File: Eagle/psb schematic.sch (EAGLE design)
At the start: 12 parts, among them J1 CONN_26X2

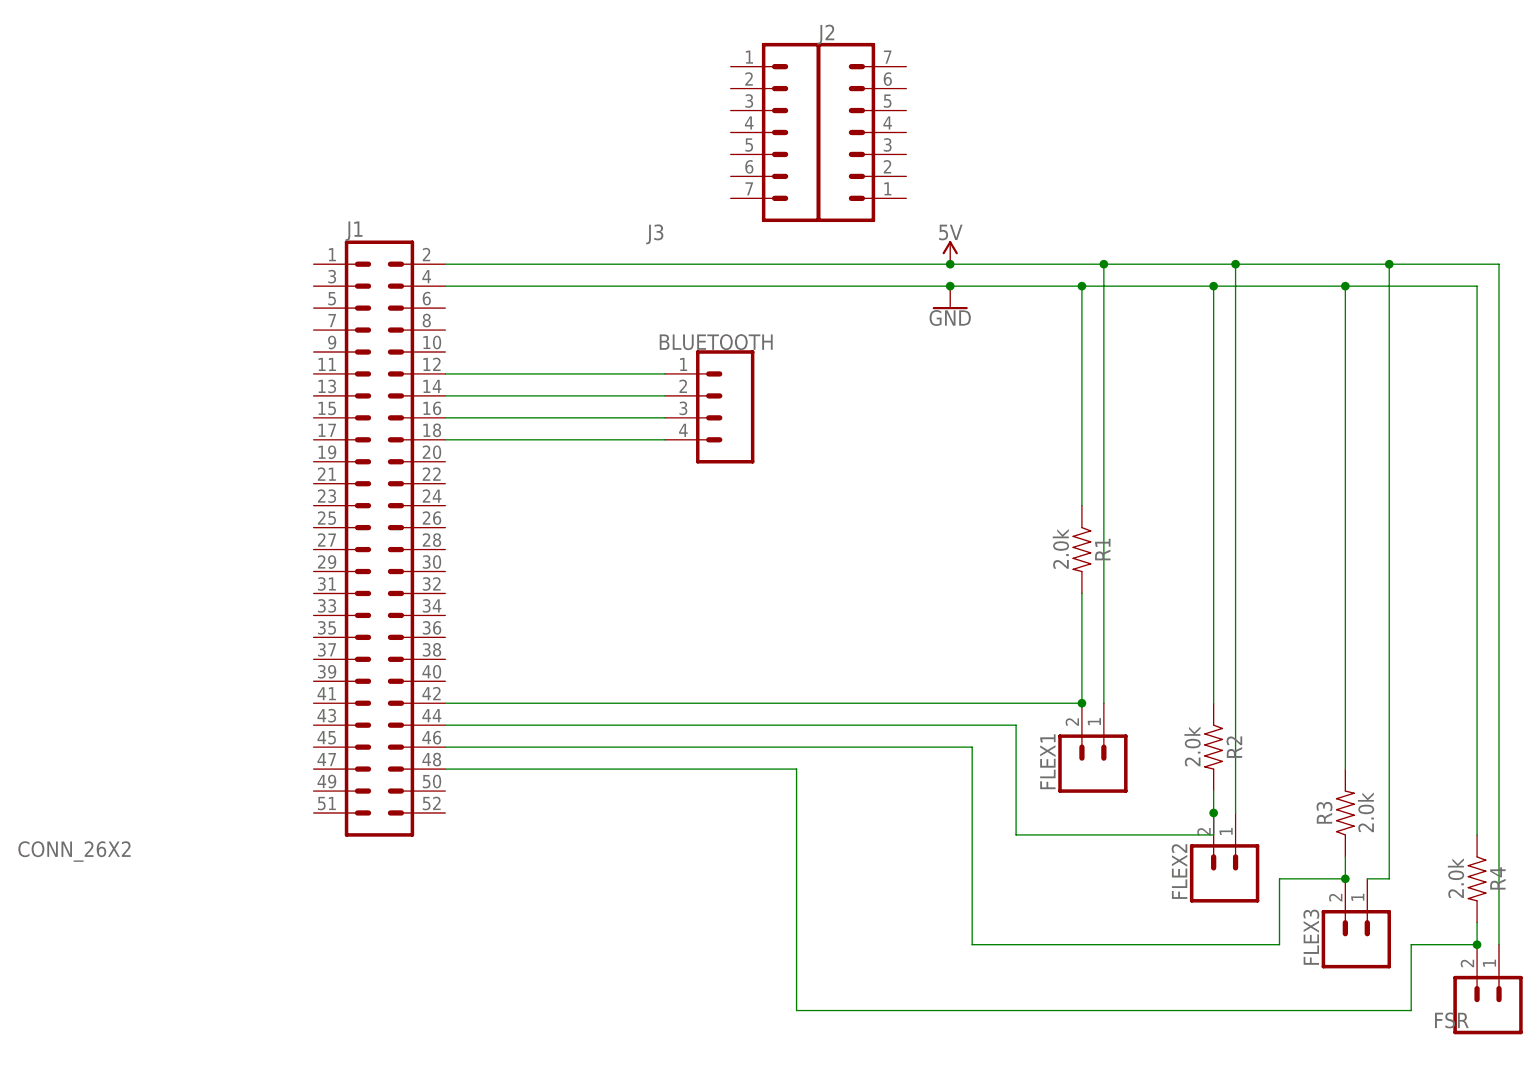
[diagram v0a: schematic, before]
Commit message: Correzioni PCB
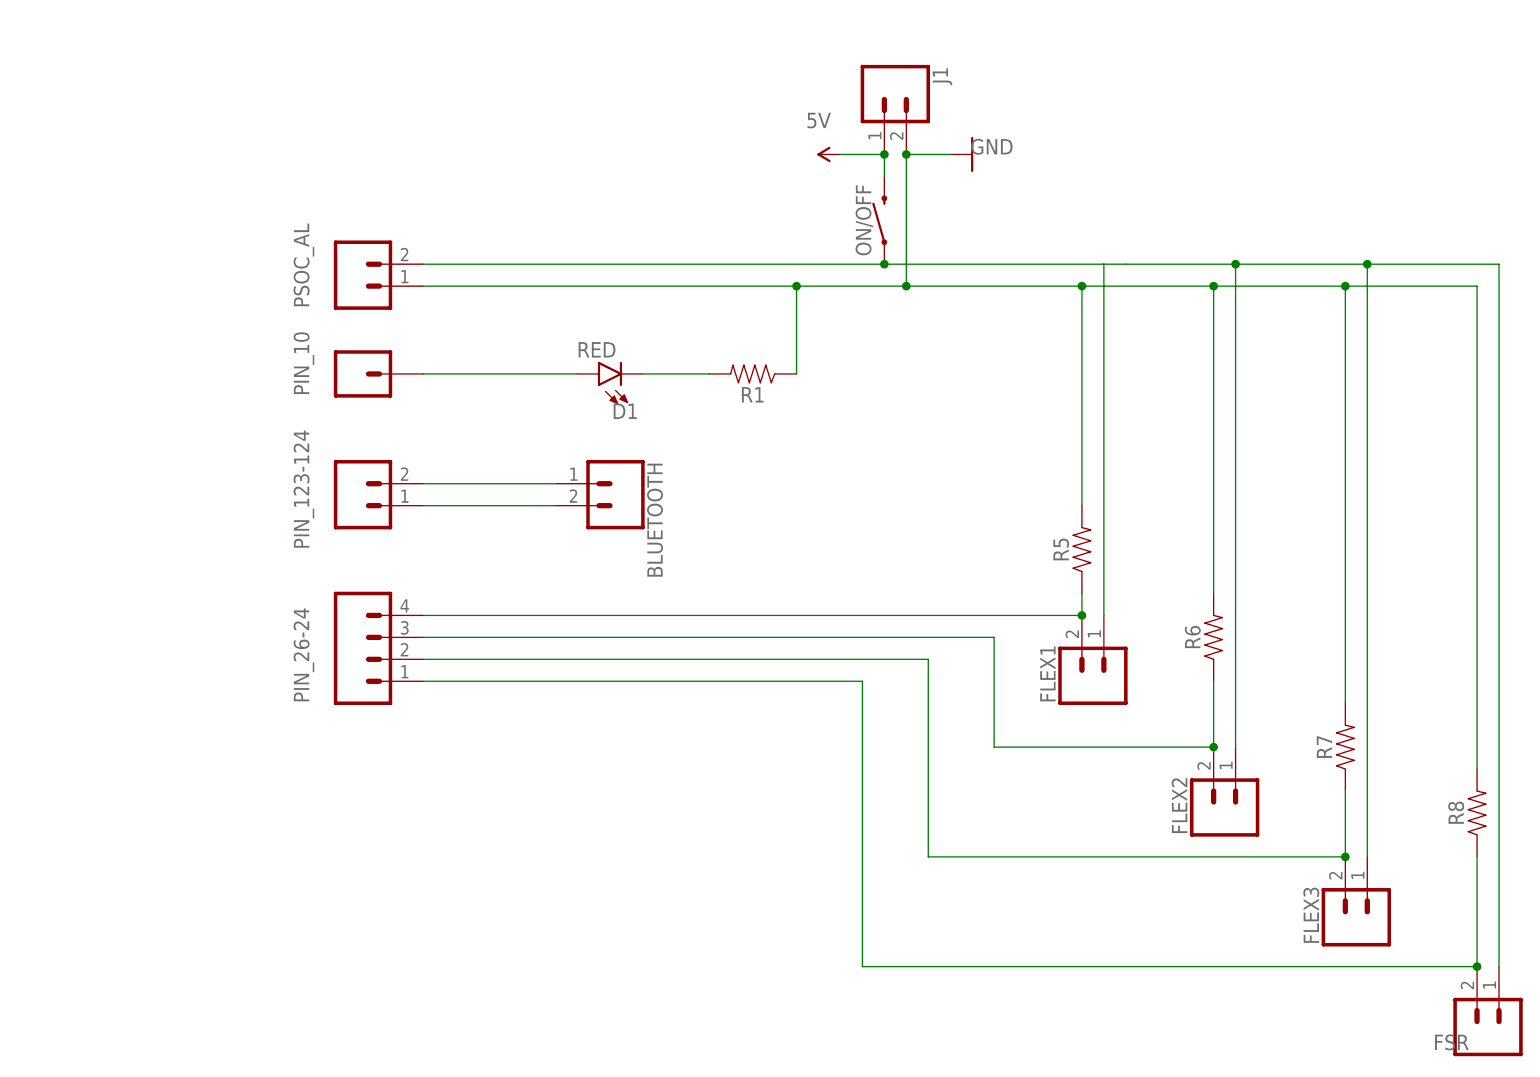
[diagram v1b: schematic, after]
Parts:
- removed J2, J3: (no value), SparkFun-Connectors:CONN_07
- removed R2, R3, R4: 2.0k, SparkFun-Resistors:2.0KOHM-0603-1/10W-5%
- added D1: RED, SparkFun-LED:LED-RED0603
- added ON/OFF: MOMENTARY-SWITCH-SPST-SMD-6.0X3.5MM, SparkFun-Switches:MOMENTARY-SWITCH-SPST-SMD-6.0X3.5MM
- added PIN_10: (no value), SparkFun-Connectors:CONN_01
- added PIN_123-124, PSOC_AL: (no value), SparkFun-Connectors:CONN_02
- added PIN_26-24: (no value), SparkFun-Connectors:CONN_04
- added R5, R6, R7, R8: (no value), SparkFun-Resistors:RESISTORAXIAL-0.3
- BLUETOOTH: device SparkFun-Connectors:CONN_04 -> SparkFun-Connectors:CONN_02
- J1: value CONN_26X2 -> (none); device SparkFun-Connectors:CONN_26X2 -> SparkFun-Connectors:CONN_02
- R1: value 2.0k -> (none); device SparkFun-Resistors:2.0KOHM-0603-1/10W-5% -> SparkFun-Resistors:RESISTORAXIAL-0.3
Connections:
- removed net N$7: BLUETOOTH.3, J1.16
- removed net N$8: BLUETOOTH.4, J1.18
- new net N$10: D1.A, PIN_10.1
- new net N$11: D1.C, R1.2
- new net N$9: FLEX1.1, FLEX2.1, FLEX3.1, FSR.1, ON/OFF.1, PSOC_AL.2
- net 5V: now also J1.1, ON/OFF.2; no longer FLEX1.1, FLEX2.1, FLEX3.1, FSR.1, J1.2
- net GND: now also J1.2, PSOC_AL.1, R5.2, R6.2, R7.2, R8.2; no longer J1.4, R2.1, R3.2, R4.1
- net N$1: now also PIN_26-24.4, R5.1; no longer J1.42, R1.2
- net N$2: now also FLEX2.2, PIN_26-24.3, R6.1; no longer FSR.2, J1.48, R4.2
- net N$3: now also FLEX3.2, PIN_26-24.2, R7.1; no longer FLEX2.2, J1.44, R2.2
- net N$4: now also PIN_123-124.2; no longer J1.12
- net N$5: now also FSR.2, PIN_26-24.1, R8.1; no longer FLEX3.2, J1.46, R3.1
- net N$6: now also PIN_123-124.1; no longer J1.14
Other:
- moved on the sheet: FLEX1, FLEX2, FLEX3, FSR, R1
